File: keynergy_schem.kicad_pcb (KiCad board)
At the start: 2 copper layers, 569.8 x 351.8 mm, 44 parts, among them J1 Conn_01x03_Pin, J2 Conn_01x03_Pin, J3 Conn_01x04_Pin, J4 Conn_01x03_Pin, J5 Conn_01x02_Pin, J6 Conn_01x03_Pin, J7 Conn_01x02_Pin, J8 Conn_01x03_Pin

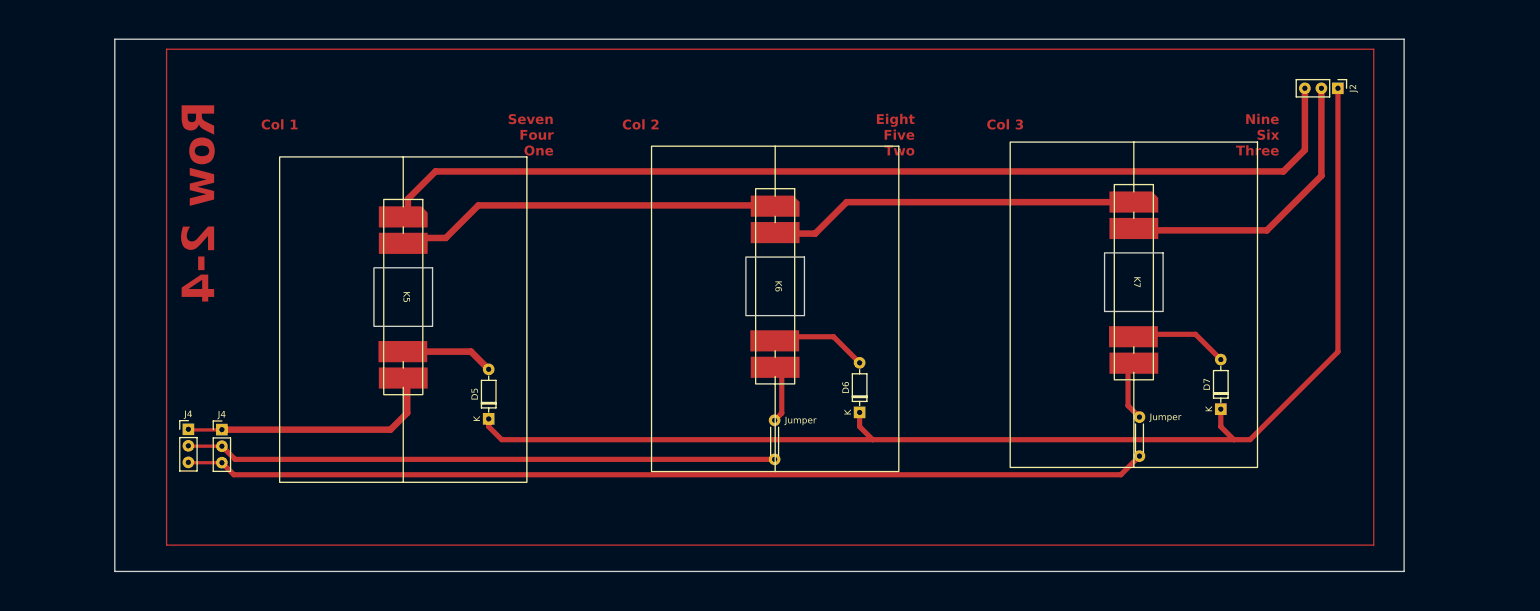
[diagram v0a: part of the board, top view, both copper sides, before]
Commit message: new updates
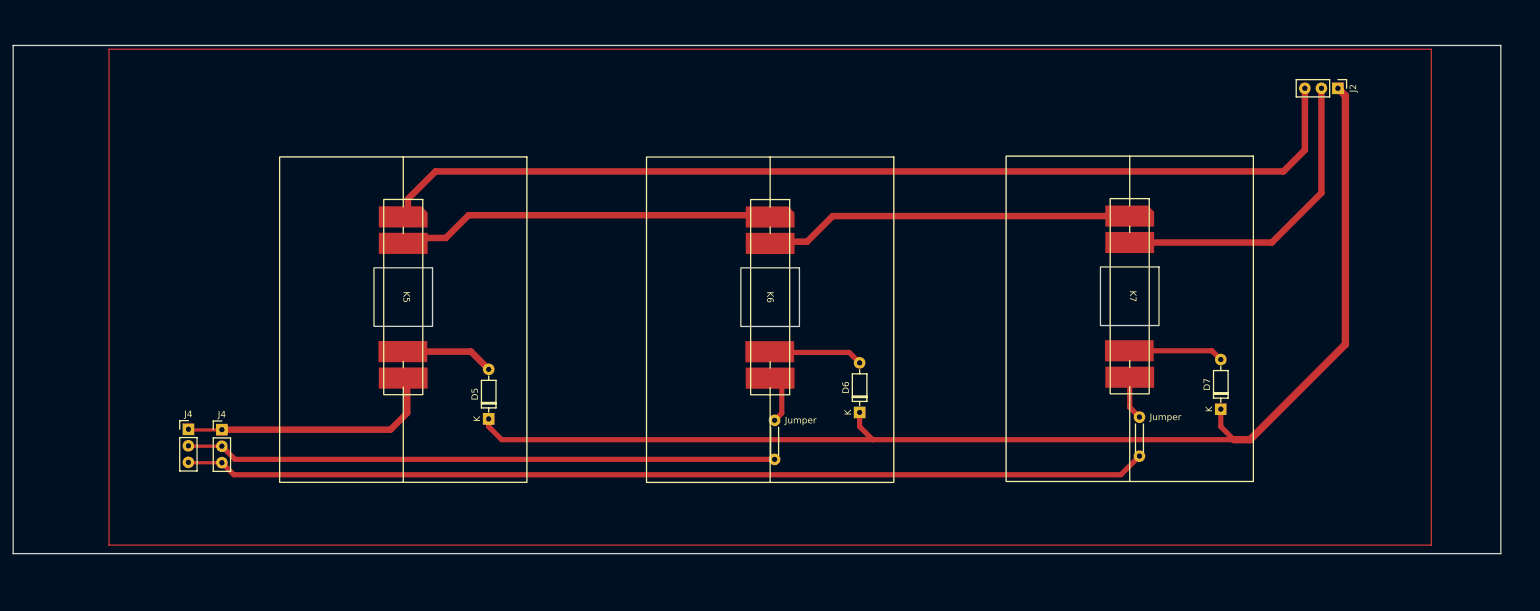
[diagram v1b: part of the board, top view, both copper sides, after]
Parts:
- moved K7 2.25 mm to (171.3, 61.7)
- moved K6 1.84 mm to (116.1, 61.9)
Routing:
- net Net-(D7-A): track 15.2 -> 11.1 mm
- net Net-(K6-C2): track 58.1 -> 54.3 mm
- net Coil 2-1: track 45.0 -> 48.7 mm
- net Col 2-3: track 158.4 -> 154.7 mm
- net Net-(D6-A): track 15.0 -> 11.9 mm
- net Col 2-2: track 99.8 -> 98.4 mm
- net Net-(K5-C2): track 58.6 -> 57.3 mm
- net Row 2: track 189.1 -> 190.1 mm
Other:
- board size 569.8 x 351.8 mm -> 585.5 x 351.8 mm
